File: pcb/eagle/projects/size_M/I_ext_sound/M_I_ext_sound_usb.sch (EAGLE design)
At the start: 19 parts

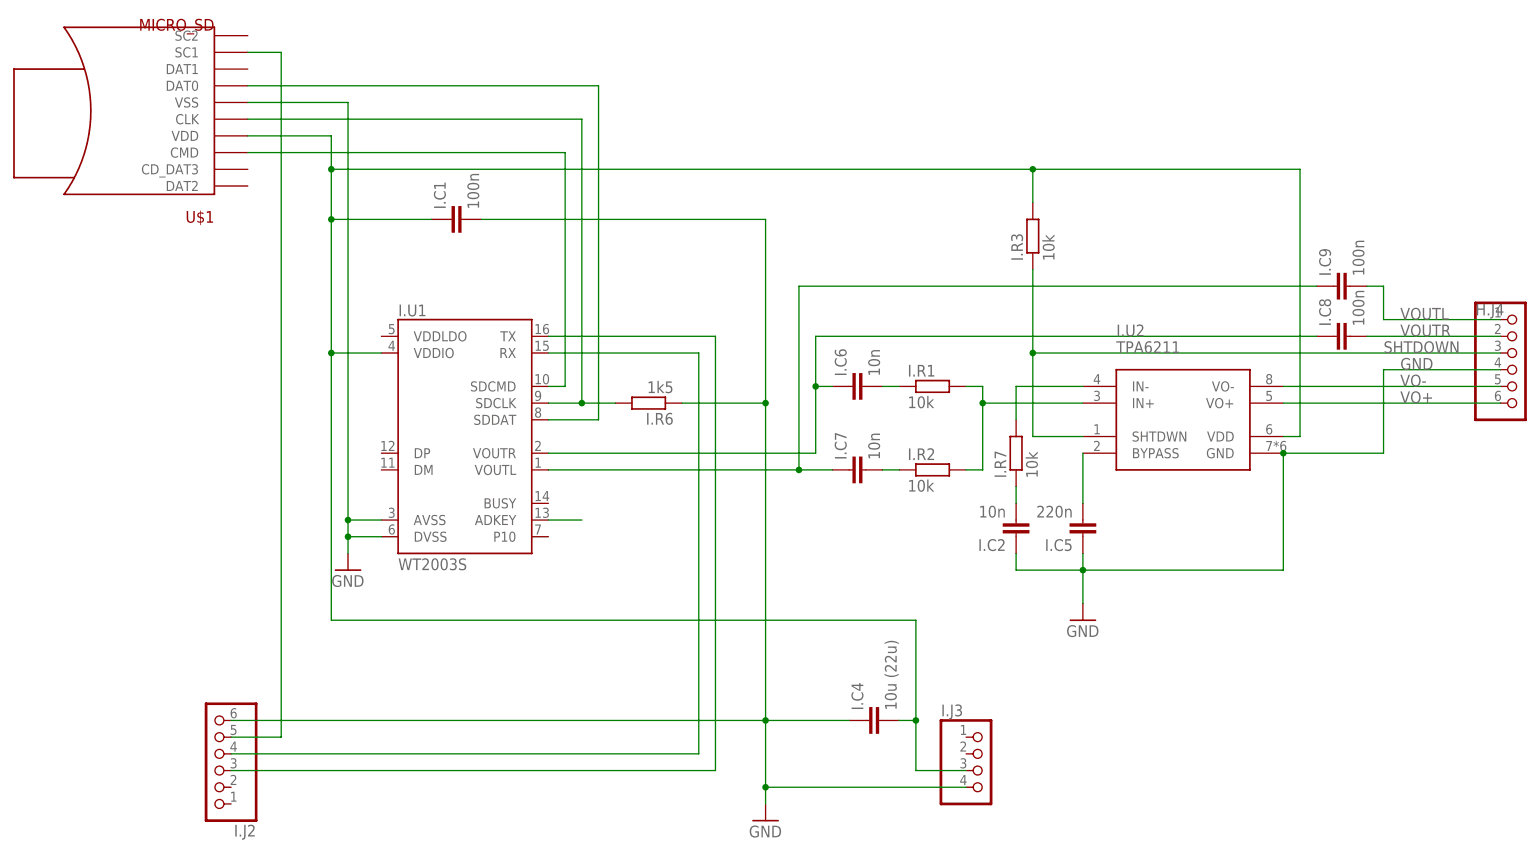
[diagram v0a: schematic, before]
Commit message: closed PCB version M.2
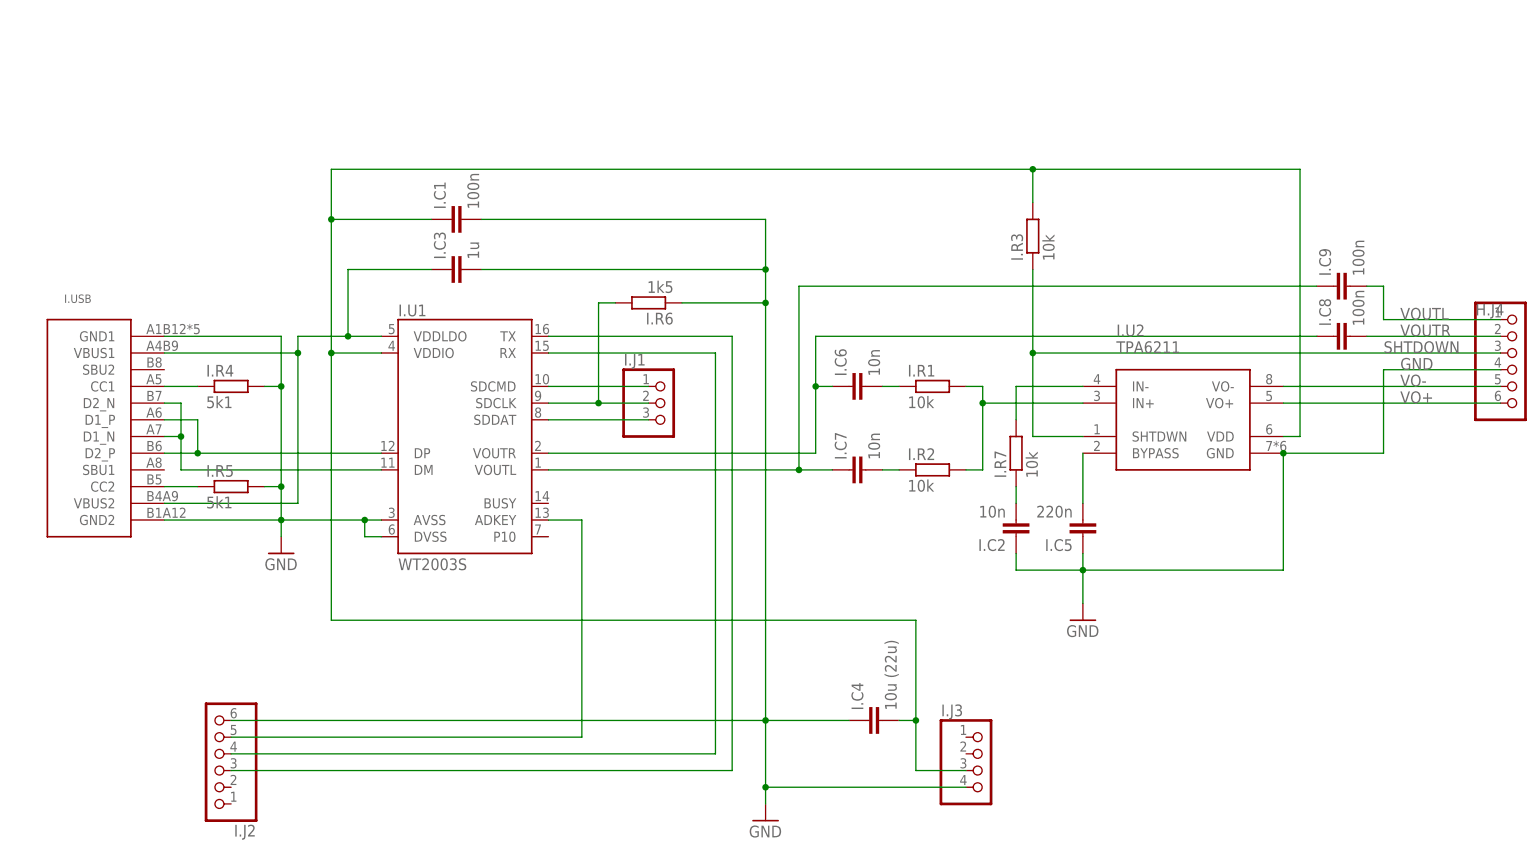
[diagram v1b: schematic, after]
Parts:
- removed U$1: MICRO_SD, hugo:MICRO_SD
- added I.C3: 1u, rcl:C-EUC0603
- added I.J1: (no value), pinhead2:PINHD-1X3
- added I.R4, I.R5: 5k1, rcl:R-EU_R0603
- added I.USB: USB-C, hugo:USB-C
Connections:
- new net N$10: I.U1.DM, I.USB.D1_N, I.USB.D2_N
- new net N$11: I.C3.1, I.U1.VDDLDO, I.USB.VBUS1, I.USB.VBUS2
- new net N$3: I.J2.5, I.U1.ADKEY
- new net N$9: I.U1.DP, I.USB.D1_P, I.USB.D2_P
- net GND: now also I.C3.2, I.R4.2, I.R5.2, I.USB.GND1, I.USB.GND2; no longer U$1.VSS
- net N$1: now also I.R5.1, I.USB.CC2; no longer I.U1.ADKEY
- net N$2: now also I.R4.1, I.USB.CC1; no longer I.J2.5, U$1.SC1
- net SDCLK: now also I.J1.2; no longer U$1.CLK
- net SDCMD: now also I.J1.1; no longer U$1.CMD
- net SDDAT: now also I.J1.3; no longer U$1.DAT0
- net VCC: no longer U$1.VDD
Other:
- moved on the sheet: I.R6
